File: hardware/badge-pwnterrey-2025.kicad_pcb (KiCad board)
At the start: 2 copper layers, 47 x 50 mm, 16 parts, among them J1 Conn_01x04_Socket, SW1 SW_RST, SW2 On, U1 PY32F002AA15M6TU

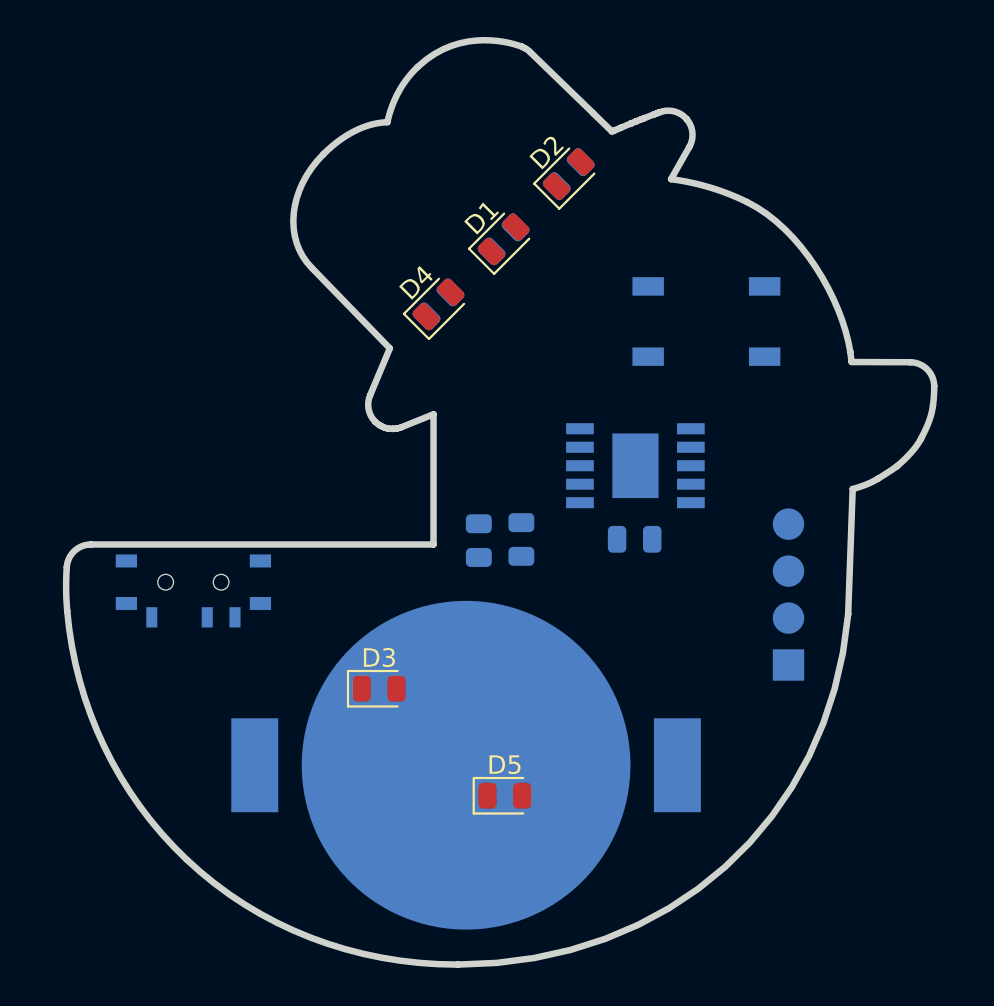
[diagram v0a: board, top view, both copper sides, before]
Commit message: feat(hw): add routes
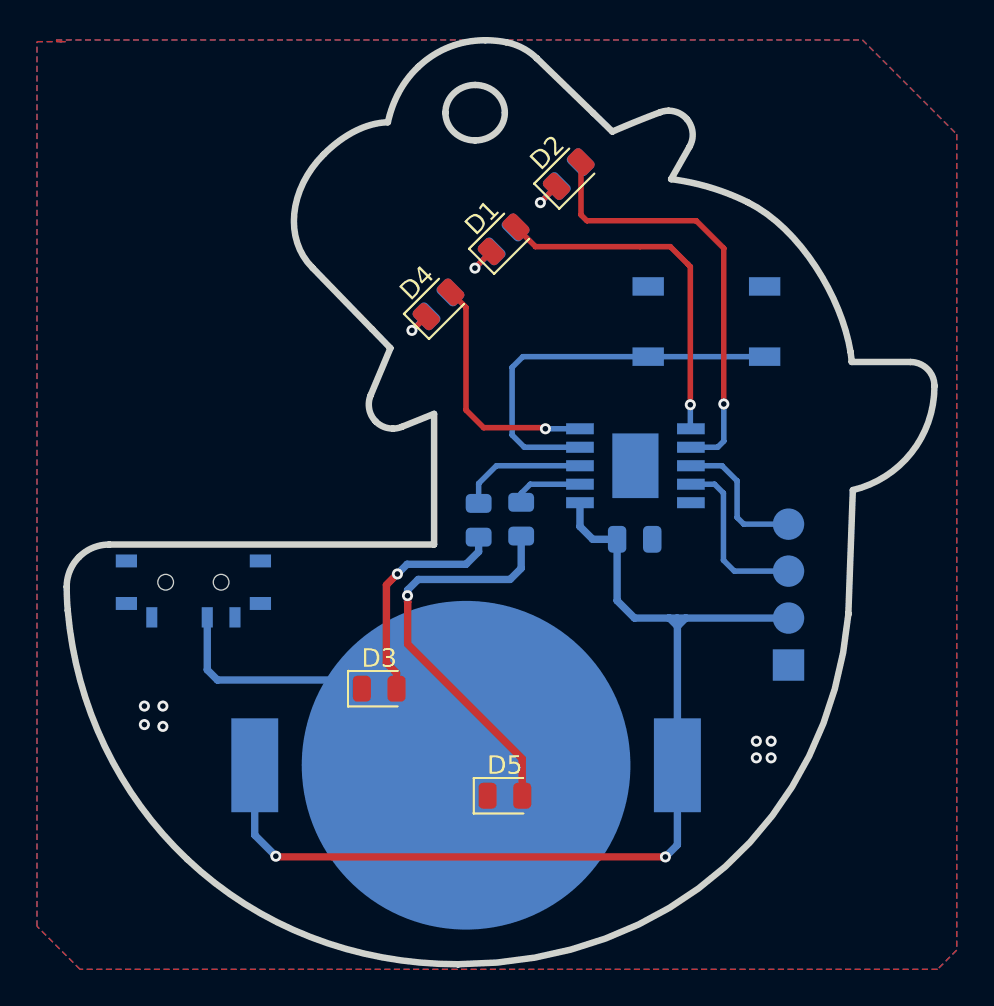
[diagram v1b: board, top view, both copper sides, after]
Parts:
- moved R5 1.10 mm to (148.0, 99.7)
- moved R3 1.10 mm to (145.7, 99.8)
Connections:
- J1 pad 2: +3V3 -> +3.3V
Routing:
- net +3.3V: track 0.00 -> 57.5 mm, vias 0 -> 2
- net /PA7: track 0.00 -> 23.7 mm, vias 0 -> 1
- net Net-(D5-A): track 0.00 -> 22.1 mm, vias 0 -> 1
- net /NRST: track 0.00 -> 21.5 mm
- net /PA6: track 0.00 -> 19.1 mm, vias 0 -> 1
- net Net-(BT1--): track 0.00 -> 19.0 mm
- net /PA1: track 0.00 -> 13.3 mm, vias 0 -> 1
- net Net-(D3-A): track 0.00 -> 12.4 mm, vias 0 -> 1
- net /SWCLK: track 0.00 -> 9.35 mm
- net /SWDIO: track 0.00 -> 7.75 mm
- net /PA5: track 0.00 -> 6.96 mm
- net /PF0: track 0.00 -> 3.87 mm
- net Net-(D1-K): track 0.00 -> 2.54 mm, vias 0 -> 1
- net Net-(D2-K): track 0.00 -> 2.51 mm, vias 0 -> 1
- net Net-(D4-K): track 0.00 -> 2.19 mm, vias 0 -> 1
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- added copper zone on B.Cu, net GND
- added copper zone on F.Cu, net GND
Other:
- board size 47 x 50 mm -> 46.9 x 50 mm
